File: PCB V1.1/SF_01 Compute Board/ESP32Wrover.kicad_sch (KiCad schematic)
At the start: 9 parts, among them J3 UART, SW3 ESP_BOOT, SW4 ESP_RESET, U28 ESP32-WROVER-E-N16R8

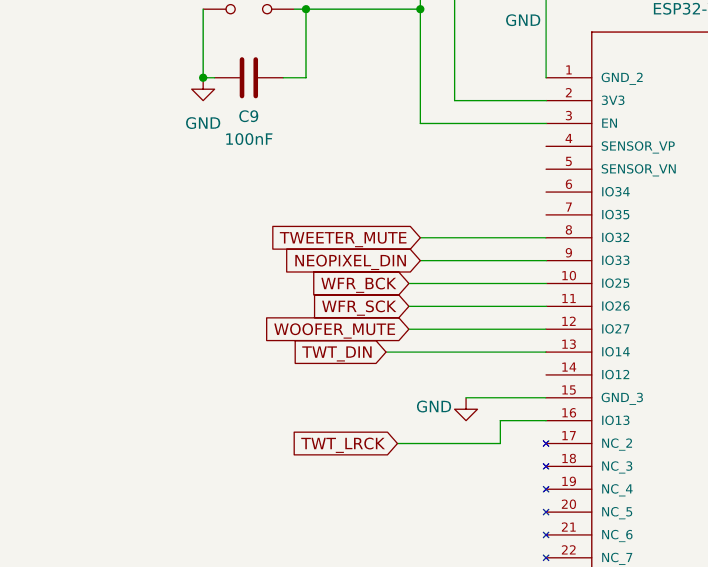
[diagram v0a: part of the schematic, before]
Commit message: Fixed minor routing issues
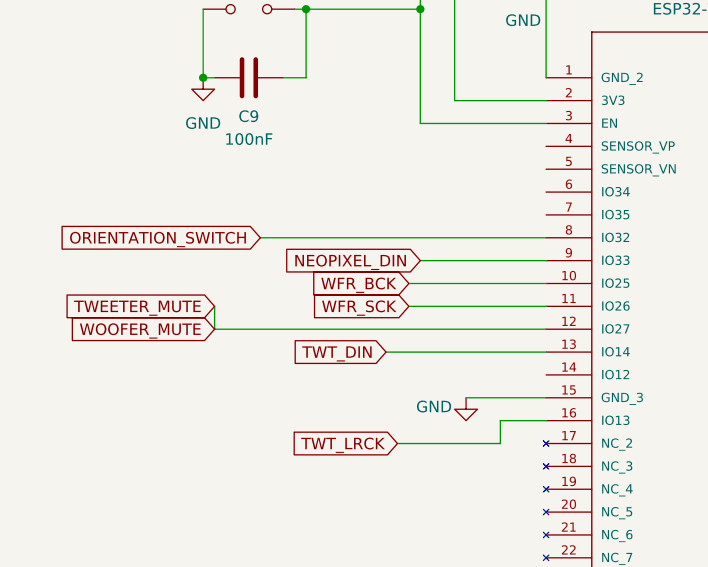
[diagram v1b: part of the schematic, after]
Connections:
- net WOOFER_MUTE is gone; now on net TWEETER_MUTE: U28.12 (IO27)
- net TWEETER_MUTE: no longer U28.8 (IO32)
- new net ORIENTATION_SWITCH: U28.8 (IO32)
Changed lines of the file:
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@@
 	(wire
 		(pts
-			(xy 60.96 83.82) (xy 74.93 83.82)
+			(xy 43.18 83.82) (xy 74.93 83.82)
 		)
 		(stroke
@@
 	(wire
 		(pts
+			(xy 38.1 91.44) (xy 38.1 93.98)
+		)
+		(stroke
+			(width 0)
+			(type default)
+		)
+	)
+	(wire
+		(pts
 			(xy 36.83 43.18) (xy 36.83 26.67)
 		)
@@
 	(wire
 		(pts
-			(xy 59.69 93.98) (xy 74.93 93.98)
+			(xy 38.1 93.98) (xy 74.93 93.98)
 		)
 		(stroke
@@
 	(global_label "TWEETER_MUTE"
 		(shape input)
-		(at 60.96 83.82 180)
-		(fields_autoplaced yes)
-		(effects
-			(font
-				(size 1.27 1.27)
-			)
-			(justify right)
-		)
-		(property "Intersheetrefs" "${INTERSHEET_REFS}"
-			(at 44.0051 83.82 0)
+		(at 38.1 91.44 180)
+		(fields_autoplaced yes)
+		(effects
+			(font
+				(size 1.27 1.27)
+			)
+			(justify right)
+		)
+		(property "Intersheetrefs" "${INTERSHEET_REFS}"
+			(at 21.1451 91.44 0)
 			(hide yes)
 			(show_name no)
@@
 	(global_label "WOOFER_MUTE"
 		(shape input)
-		(at 59.69 93.98 180)
-		(fields_autoplaced yes)
-		(effects
-			(font
-				(size 1.27 1.27)
-			)
-			(justify right)
-		)
-		(property "Intersheetrefs" "${INTERSHEET_REFS}"
-			(at 43.2187 93.98 0)
+		(at 38.1 93.98 180)
+		(fields_autoplaced yes)
+		(effects
+			(font
+				(size 1.27 1.27)
+			)
+			(justify right)
+		)
+		(property "Intersheetrefs" "${INTERSHEET_REFS}"
+			(at 21.6287 93.98 0)
 			(hide yes)
 			(show_name no)
@@
 			)
 		)
+	)
+	(global_label "ORIENTATION_SWITCH"
+		(shape input)
+		(at 43.18 83.82 180)
+		(fields_autoplaced yes)
+		(effects
+			(font
+				(size 1.27 1.27)
+			)
+			(justify right)
+		)
+		(property "Intersheetrefs" "${INTERSHEET_REFS}"
+			(at 20.419 83.82 0)
+			(hide yes)
+			(show_name no)
+			(do_not_autoplace no)
+			(effects
+				(font
+					(size 1.27 1.27)
+				)
+				(justify right)
+			)
+		)
